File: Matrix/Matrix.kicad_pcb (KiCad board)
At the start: 4 copper layers, 81 x 49.8 mm, 513 parts, among them J1 Conn_02x24_Odd_Even

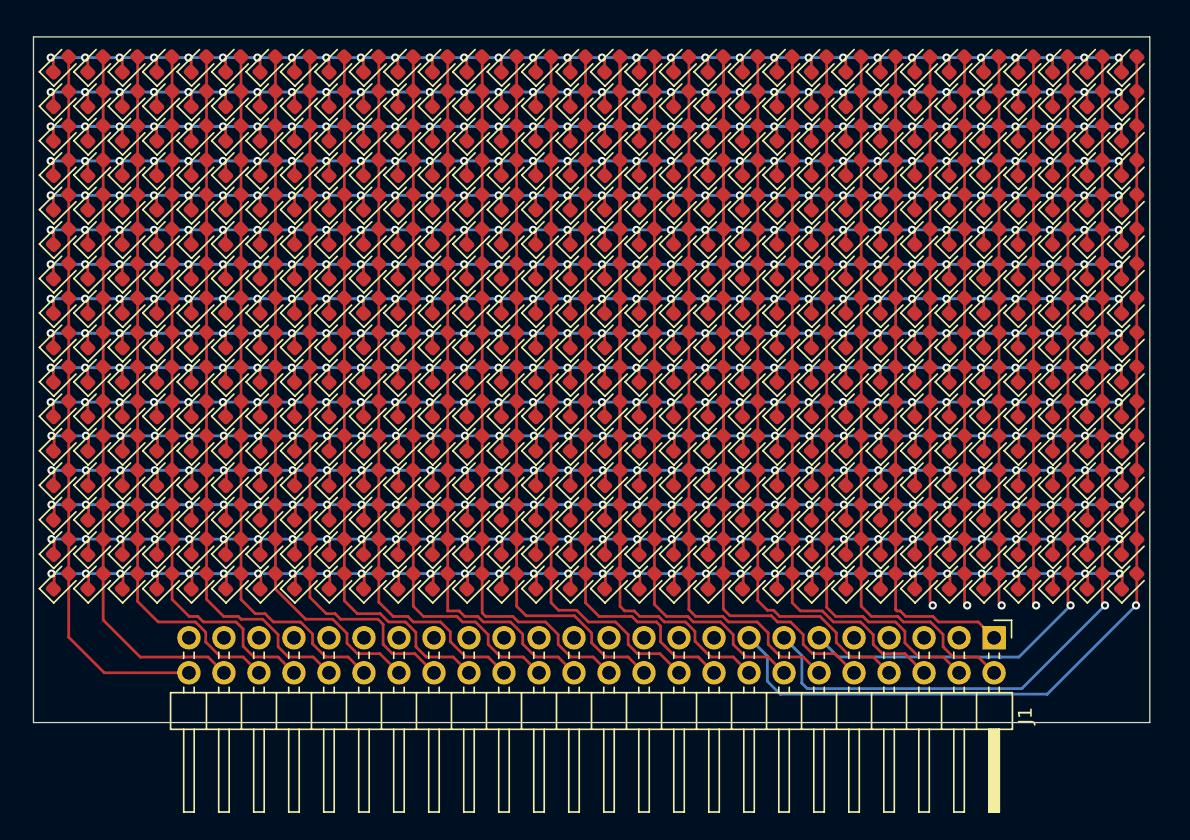
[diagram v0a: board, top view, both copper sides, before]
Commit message: getting ready for another review
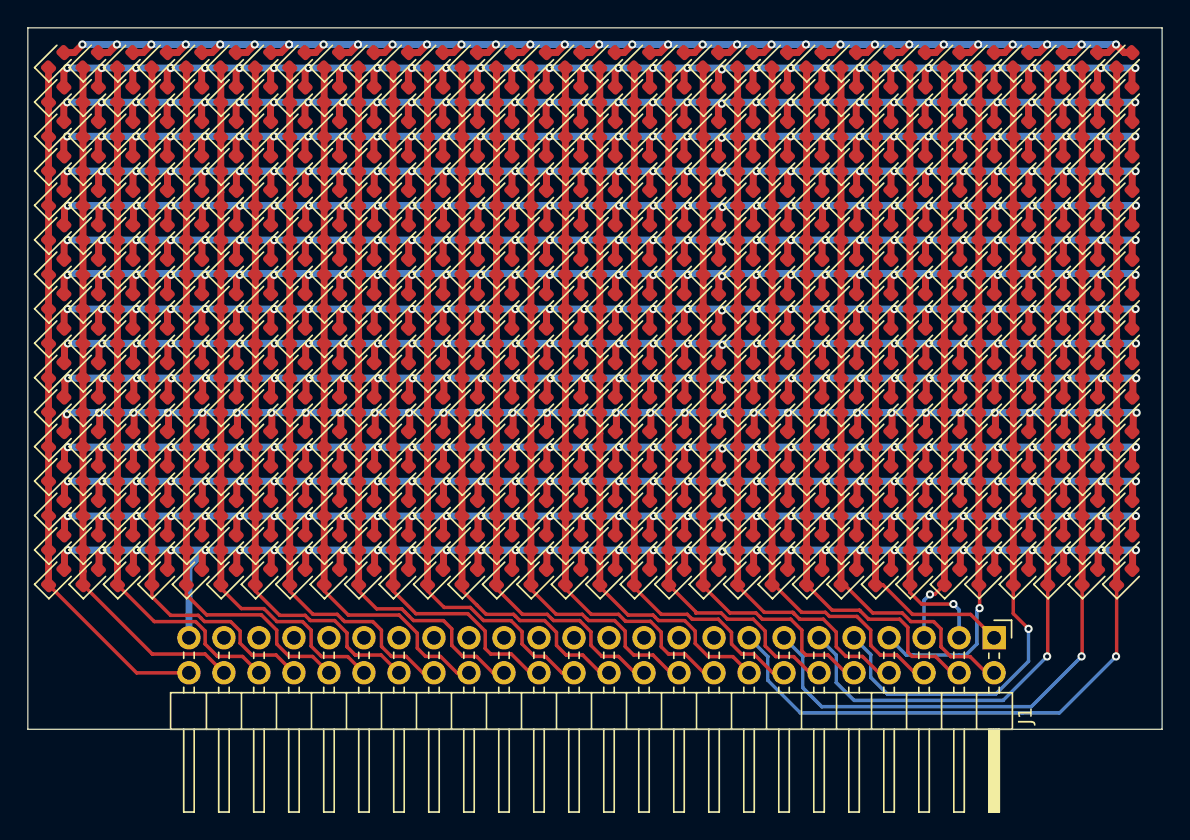
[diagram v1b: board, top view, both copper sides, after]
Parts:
- D1, D10, D100, D101, D102, D103, D104, D105, D106, D107, D108, D109, D11, D110, D111, D112, D113, D114, D115, D116, D117, D118, D119, D12, D120, D121, D122, D123, D124, D125, D126, D127, D128, D129, D13, D130, D131, D132, D133, D134, D135, D136, D137, D138, D139, D14, D140, D141, D142, D143, D144, D145, D146, D147, D148, D149, D15, D150, D151, D152, D153, D154, D155, D156, D157, D158, D159, D16, D160, D161, D162, D163, D164, D165, D166, D167, D168, D169, D17, D170, D171, D172, D173, D174, D175, D176, D177, D178, D179, D18, D180, D181, D182, D183, D184, D185, D186, D187, D188, D189, D19, D190, D191, D192, D193, D194, D195, D196, D197, D198, D199, D2, D20, D200, D201, D202, D203, D204, D205, D206, D207, D208, D209, D21, D210, D211, D212, D213, D214, D215, D216, D217, D218, D219, D22, D220, D221, D222, D223, D224, D225, D226, D227, D228, D229, D23, D230, D231, D232, D233, D234, D235, D236, D237, D238, D239, D24, D240, D241, D242, D243, D244, D245, D246, D247, D248, D249, D25, D250, D251, D252, D253, D254, D255, D256, D257, D258, D259, D26, D260, D261, D262, D263, D264, D265, D266, D267, D268, D269, D27, D270, D271, D272, D273, D274, D275, D276, D277, D278, D279, D28, D280, D281, D282, D283, D284, D285, D286, D287, D288, D289, D29, D290, D291, D292, D293, D294, D295, D296, D297, D298, D299, D3, D30, D300, D301, D302, D303, D304, D305, D306, D307, D308, D309, D31, D310, D311, D312, D313, D314, D315, D316, D317, D318, D319, D32, D320, D321, D322, D323, D324, D325, D326, D327, D328, D329, D33, D330, D331, D332, D333, D334, D335, D336, D337, D338, D339, D34, D340, D341, D342, D343, D344, D345, D346, D347, D348, D349, D35, D350, D351, D352, D353, D354, D355, D356, D357, D358, D359, D36, D360, D361, D362, D363, D364, D365, D366, D367, D368, D369, D37, D370, D371, D372, D373, D374, D375, D376, D377, D378, D379, D38, D380, D381, D382, D383, D384, D385, D386, D387, D388, D389, D39, D390, D391, D392, D393, D394, D395, D396, D397, D398, D399, D4, D40, D400, D401, D402, D403, D404, D405, D406, D407, D408, D409, D41, D410, D411, D412, D413, D414, D415, D416, D417, D418, D419, D42, D420, D421, D422, D423, D424, D425, D426, D427, D428, D429, D43, D430, D431, D432, D433, D434, D435, D436, D437, D438, D439, D44, D440, D441, D442, D443, D444, D445, D446, D447, D448, D449, D45, D450, D451, D452, D453, D454, D455, D456, D457, D458, D459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: value LED -> SML-D12U1WT86
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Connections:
- D10 pad 1: Net-(D10-K) -> Net-(D1-K)
- D10 pad 2: Net-(D1-A) -> Net-(D10-A)
- D101 pad 1: Net-(D101-K) -> Net-(D100-K)
- D101 pad 2: Net-(D100-A) -> Net-(D101-A)
- D102 pad 1: Net-(D102-K) -> Net-(D100-K)
- D102 pad 2: Net-(D100-A) -> Net-(D102-A)
- D103 pad 1: Net-(D103-K) -> Net-(D100-K)
- D103 pad 2: Net-(D100-A) -> Net-(D103-A)
- D104 pad 1: Net-(D104-K) -> Net-(D100-K)
- D104 pad 2: Net-(D100-A) -> Net-(D104-A)
- D105 pad 1: Net-(D105-K) -> Net-(D100-K)
- D105 pad 2: Net-(D100-A) -> Net-(D105-A)
- D106 pad 1: Net-(D10-K) -> Net-(D100-K)
- D106 pad 2: Net-(D100-A) -> Net-(D10-A)
- D107 pad 1: Net-(D107-K) -> Net-(D100-K)
- D107 pad 2: Net-(D100-A) -> Net-(D107-A)
- D108 pad 1: Net-(D108-K) -> Net-(D100-K)
- D108 pad 2: Net-(D100-A) -> Net-(D108-A)
- D109 pad 1: Net-(D109-K) -> Net-(D100-K)
- D109 pad 2: Net-(D100-A) -> Net-(D109-A)
- D11 pad 1: Net-(D107-K) -> Net-(D1-K)
- D11 pad 2: Net-(D1-A) -> Net-(D107-A)
- D110 pad 1: Net-(D110-K) -> Net-(D100-K)
- D110 pad 2: Net-(D100-A) -> Net-(D110-A)
- D111 pad 1: Net-(D111-K) -> Net-(D100-K)
- D111 pad 2: Net-(D100-A) -> Net-(D111-A)
- D112 pad 1: Net-(D112-K) -> Net-(D100-K)
- D112 pad 2: Net-(D100-A) -> Net-(D112-A)
- D113 pad 1: Net-(D1-K) -> Net-(D113-K)
- D113 pad 2: Net-(D113-A) -> Net-(D1-A)
- D114 pad 1: Net-(D114-K) -> Net-(D113-K)
- D114 pad 2: Net-(D113-A) -> Net-(D114-A)
- D115 pad 1: Net-(D115-K) -> Net-(D113-K)
- D115 pad 2: Net-(D113-A) -> Net-(D115-A)
- D116 pad 1: Net-(D100-K) -> Net-(D113-K)
- D116 pad 2: Net-(D113-A) -> Net-(D100-A)
- D117 pad 1: Net-(D101-K) -> Net-(D113-K)
- D117 pad 2: Net-(D113-A) -> Net-(D101-A)
- D118 pad 1: Net-(D102-K) -> Net-(D113-K)
- D118 pad 2: Net-(D113-A) -> Net-(D102-A)
- D119 pad 1: Net-(D103-K) -> Net-(D113-K)
- D119 pad 2: Net-(D113-A) -> Net-(D103-A)
- D12 pad 1: Net-(D108-K) -> Net-(D1-K)
- D12 pad 2: Net-(D1-A) -> Net-(D108-A)
- D120 pad 1: Net-(D104-K) -> Net-(D113-K)
- D120 pad 2: Net-(D113-A) -> Net-(D104-A)
- D121 pad 1: Net-(D105-K) -> Net-(D113-K)
- D121 pad 2: Net-(D113-A) -> Net-(D105-A)
- D122 pad 1: Net-(D10-K) -> Net-(D113-K)
- D122 pad 2: Net-(D113-A) -> Net-(D10-A)
- D123 pad 1: Net-(D107-K) -> Net-(D113-K)
- D123 pad 2: Net-(D113-A) -> Net-(D107-A)
- D124 pad 1: Net-(D108-K) -> Net-(D113-K)
- D124 pad 2: Net-(D113-A) -> Net-(D108-A)
- D125 pad 1: Net-(D109-K) -> Net-(D113-K)
- D125 pad 2: Net-(D113-A) -> Net-(D109-A)
- D126 pad 1: Net-(D110-K) -> Net-(D113-K)
- D126 pad 2: Net-(D113-A) -> Net-(D110-A)
- D127 pad 1: Net-(D111-K) -> Net-(D113-K)
- D127 pad 2: Net-(D113-A) -> Net-(D111-A)
- D128 pad 1: Net-(D112-K) -> Net-(D113-K)
- D128 pad 2: Net-(D113-A) -> Net-(D112-A)
- D129 pad 1: Net-(D1-K) -> Net-(D129-K)
- D129 pad 2: Net-(D129-A) -> Net-(D1-A)
- D13 pad 1: Net-(D109-K) -> Net-(D1-K)
- D13 pad 2: Net-(D1-A) -> Net-(D109-A)
- D130 pad 1: Net-(D114-K) -> Net-(D129-K)
- D130 pad 2: Net-(D129-A) -> Net-(D114-A)
- D131 pad 1: Net-(D115-K) -> Net-(D129-K)
- D131 pad 2: Net-(D129-A) -> Net-(D115-A)
- D132 pad 1: Net-(D100-K) -> Net-(D129-K)
- D132 pad 2: Net-(D129-A) -> Net-(D100-A)
- D133 pad 1: Net-(D101-K) -> Net-(D129-K)
- D133 pad 2: Net-(D129-A) -> Net-(D101-A)
- D134 pad 1: Net-(D102-K) -> Net-(D129-K)
- D134 pad 2: Net-(D129-A) -> Net-(D102-A)
- D135 pad 1: Net-(D103-K) -> Net-(D129-K)
- D135 pad 2: Net-(D129-A) -> Net-(D103-A)
- D136 pad 1: Net-(D104-K) -> Net-(D129-K)
- D136 pad 2: Net-(D129-A) -> Net-(D104-A)
- D137 pad 1: Net-(D105-K) -> Net-(D129-K)
- D137 pad 2: Net-(D129-A) -> Net-(D105-A)
- D138 pad 1: Net-(D10-K) -> Net-(D129-K)
- D138 pad 2: Net-(D129-A) -> Net-(D10-A)
- D139 pad 1: Net-(D107-K) -> Net-(D129-K)
- D139 pad 2: Net-(D129-A) -> Net-(D107-A)
- D14 pad 1: Net-(D110-K) -> Net-(D1-K)
- D14 pad 2: Net-(D1-A) -> Net-(D110-A)
- D140 pad 1: Net-(D108-K) -> Net-(D129-K)
- D140 pad 2: Net-(D129-A) -> Net-(D108-A)
- D141 pad 1: Net-(D109-K) -> Net-(D129-K)
- D141 pad 2: Net-(D129-A) -> Net-(D109-A)
- D142 pad 1: Net-(D110-K) -> Net-(D129-K)
- D142 pad 2: Net-(D129-A) -> Net-(D110-A)
- D143 pad 1: Net-(D111-K) -> Net-(D129-K)
- D143 pad 2: Net-(D129-A) -> Net-(D111-A)
- D144 pad 1: Net-(D112-K) -> Net-(D129-K)
- D144 pad 2: Net-(D129-A) -> Net-(D112-A)
- D145 pad 1: Net-(D1-K) -> Net-(D145-K)
- D145 pad 2: Net-(D145-A) -> Net-(D1-A)
- D146 pad 1: Net-(D114-K) -> Net-(D145-K)
- D146 pad 2: Net-(D145-A) -> Net-(D114-A)
- D147 pad 1: Net-(D115-K) -> Net-(D145-K)
- D147 pad 2: Net-(D145-A) -> Net-(D115-A)
- D148 pad 1: Net-(D100-K) -> Net-(D145-K)
- D148 pad 2: Net-(D145-A) -> Net-(D100-A)
- D149 pad 1: Net-(D101-K) -> Net-(D145-K)
- D149 pad 2: Net-(D145-A) -> Net-(D101-A)
- D15 pad 1: Net-(D111-K) -> Net-(D1-K)
- D15 pad 2: Net-(D1-A) -> Net-(D111-A)
- D150 pad 1: Net-(D102-K) -> Net-(D145-K)
- D150 pad 2: Net-(D145-A) -> Net-(D102-A)
- D151 pad 1: Net-(D103-K) -> Net-(D145-K)
- D151 pad 2: Net-(D145-A) -> Net-(D103-A)
- D152 pad 1: Net-(D104-K) -> Net-(D145-K)
- D152 pad 2: Net-(D145-A) -> Net-(D104-A)
- D153 pad 1: Net-(D105-K) -> Net-(D145-K)
- D153 pad 2: Net-(D145-A) -> Net-(D105-A)
- D154 pad 1: Net-(D10-K) -> Net-(D145-K)
- D154 pad 2: Net-(D145-A) -> Net-(D10-A)
- D155 pad 1: Net-(D107-K) -> Net-(D145-K)
- D155 pad 2: Net-(D145-A) -> Net-(D107-A)
- D156 pad 1: Net-(D108-K) -> Net-(D145-K)
- D156 pad 2: Net-(D145-A) -> Net-(D108-A)
- D157 pad 1: Net-(D109-K) -> Net-(D145-K)
- D157 pad 2: Net-(D145-A) -> Net-(D109-A)
- D158 pad 1: Net-(D110-K) -> Net-(D145-K)
- D158 pad 2: Net-(D145-A) -> Net-(D110-A)
- D159 pad 1: Net-(D111-K) -> Net-(D145-K)
- D159 pad 2: Net-(D145-A) -> Net-(D111-A)
- D16 pad 1: Net-(D112-K) -> Net-(D1-K)
- D16 pad 2: Net-(D1-A) -> Net-(D112-A)
- D160 pad 1: Net-(D112-K) -> Net-(D145-K)
- D160 pad 2: Net-(D145-A) -> Net-(D112-A)
- D161 pad 1: Net-(D1-K) -> Net-(D161-K)
- D161 pad 2: Net-(D161-A) -> Net-(D1-A)
- D162 pad 1: Net-(D114-K) -> Net-(D161-K)
- D162 pad 2: Net-(D161-A) -> Net-(D114-A)
- D163 pad 1: Net-(D115-K) -> Net-(D161-K)
- D163 pad 2: Net-(D161-A) -> Net-(D115-A)
- D164 pad 1: Net-(D100-K) -> Net-(D161-K)
- D164 pad 2: Net-(D161-A) -> Net-(D100-A)
- D165 pad 1: Net-(D101-K) -> Net-(D161-K)
- D165 pad 2: Net-(D161-A) -> Net-(D101-A)
- D166 pad 1: Net-(D102-K) -> Net-(D161-K)
- D166 pad 2: Net-(D161-A) -> Net-(D102-A)
- D167 pad 1: Net-(D103-K) -> Net-(D161-K)
- D167 pad 2: Net-(D161-A) -> Net-(D103-A)
- D168 pad 1: Net-(D104-K) -> Net-(D161-K)
- D168 pad 2: Net-(D161-A) -> Net-(D104-A)
- D169 pad 1: Net-(D105-K) -> Net-(D161-K)
- D169 pad 2: Net-(D161-A) -> Net-(D105-A)
- D17 pad 1: Net-(D1-K) -> Net-(D17-K)
- D17 pad 2: Net-(D17-A) -> Net-(D1-A)
- D170 pad 1: Net-(D10-K) -> Net-(D161-K)
- D170 pad 2: Net-(D161-A) -> Net-(D10-A)
- D171 pad 1: Net-(D107-K) -> Net-(D161-K)
- D171 pad 2: Net-(D161-A) -> Net-(D107-A)
- D172 pad 1: Net-(D108-K) -> Net-(D161-K)
- D172 pad 2: Net-(D161-A) -> Net-(D108-A)
- D173 pad 1: Net-(D109-K) -> Net-(D161-K)
- D173 pad 2: Net-(D161-A) -> Net-(D109-A)
- D174 pad 1: Net-(D110-K) -> Net-(D161-K)
- D174 pad 2: Net-(D161-A) -> Net-(D110-A)
- D175 pad 1: Net-(D111-K) -> Net-(D161-K)
- D175 pad 2: Net-(D161-A) -> Net-(D111-A)
- D176 pad 1: Net-(D112-K) -> Net-(D161-K)
- D176 pad 2: Net-(D161-A) -> Net-(D112-A)
- D177 pad 1: Net-(D1-K) -> Net-(D177-K)
- D177 pad 2: Net-(D177-A) -> Net-(D1-A)
- D178 pad 1: Net-(D114-K) -> Net-(D177-K)
- D178 pad 2: Net-(D177-A) -> Net-(D114-A)
- D179 pad 1: Net-(D115-K) -> Net-(D177-K)
- D179 pad 2: Net-(D177-A) -> Net-(D115-A)
- D18 pad 1: Net-(D114-K) -> Net-(D17-K)
- D18 pad 2: Net-(D17-A) -> Net-(D114-A)
- D180 pad 1: Net-(D100-K) -> Net-(D177-K)
- D180 pad 2: Net-(D177-A) -> Net-(D100-A)
- D181 pad 1: Net-(D101-K) -> Net-(D177-K)
- D181 pad 2: Net-(D177-A) -> Net-(D101-A)
- D182 pad 1: Net-(D102-K) -> Net-(D177-K)
- D182 pad 2: Net-(D177-A) -> Net-(D102-A)
- D183 pad 1: Net-(D103-K) -> Net-(D177-K)
- D183 pad 2: Net-(D177-A) -> Net-(D103-A)
- D184 pad 1: Net-(D104-K) -> Net-(D177-K)
- D184 pad 2: Net-(D177-A) -> Net-(D104-A)
- D185 pad 1: Net-(D105-K) -> Net-(D177-K)
- D185 pad 2: Net-(D177-A) -> Net-(D105-A)
- D186 pad 1: Net-(D10-K) -> Net-(D177-K)
- D186 pad 2: Net-(D177-A) -> Net-(D10-A)
- D187 pad 1: Net-(D107-K) -> Net-(D177-K)
- D187 pad 2: Net-(D177-A) -> Net-(D107-A)
- D188 pad 1: Net-(D108-K) -> Net-(D177-K)
- D188 pad 2: Net-(D177-A) -> Net-(D108-A)
- D189 pad 1: Net-(D109-K) -> Net-(D177-K)
- D189 pad 2: Net-(D177-A) -> Net-(D109-A)
- D19 pad 1: Net-(D115-K) -> Net-(D17-K)
- D19 pad 2: Net-(D17-A) -> Net-(D115-A)
- D190 pad 1: Net-(D110-K) -> Net-(D177-K)
- D190 pad 2: Net-(D177-A) -> Net-(D110-A)
- D191 pad 1: Net-(D111-K) -> Net-(D177-K)
- D191 pad 2: Net-(D177-A) -> Net-(D111-A)
- D192 pad 1: Net-(D112-K) -> Net-(D177-K)
- D192 pad 2: Net-(D177-A) -> Net-(D112-A)
- D193 pad 1: Net-(D1-K) -> Net-(D193-K)
- D193 pad 2: Net-(D193-A) -> Net-(D1-A)
- D194 pad 1: Net-(D114-K) -> Net-(D193-K)
- D194 pad 2: Net-(D193-A) -> Net-(D114-A)
- D195 pad 1: Net-(D115-K) -> Net-(D193-K)
- D195 pad 2: Net-(D193-A) -> Net-(D115-A)
- D196 pad 1: Net-(D100-K) -> Net-(D193-K)
- D196 pad 2: Net-(D193-A) -> Net-(D100-A)
- D197 pad 1: Net-(D101-K) -> Net-(D193-K)
- D197 pad 2: Net-(D193-A) -> Net-(D101-A)
- D198 pad 1: Net-(D102-K) -> Net-(D193-K)
- D198 pad 2: Net-(D193-A) -> Net-(D102-A)
- D199 pad 1: Net-(D103-K) -> Net-(D193-K)
- D199 pad 2: Net-(D193-A) -> Net-(D103-A)
- D2 pad 1: Net-(D114-K) -> Net-(D1-K)
- D2 pad 2: Net-(D1-A) -> Net-(D114-A)
- D20 pad 1: Net-(D100-K) -> Net-(D17-K)
- D20 pad 2: Net-(D17-A) -> Net-(D100-A)
- D200 pad 1: Net-(D104-K) -> Net-(D193-K)
- D200 pad 2: Net-(D193-A) -> Net-(D104-A)
- D201 pad 1: Net-(D105-K) -> Net-(D193-K)
- D201 pad 2: Net-(D193-A) -> Net-(D105-A)
- D202 pad 1: Net-(D10-K) -> Net-(D193-K)
- D202 pad 2: Net-(D193-A) -> Net-(D10-A)
- D203 pad 1: Net-(D107-K) -> Net-(D193-K)
- D203 pad 2: Net-(D193-A) -> Net-(D107-A)
- D204 pad 1: Net-(D108-K) -> Net-(D193-K)
- D204 pad 2: Net-(D193-A) -> Net-(D108-A)
- D205 pad 1: Net-(D109-K) -> Net-(D193-K)
- D205 pad 2: Net-(D193-A) -> Net-(D109-A)
- D206 pad 1: Net-(D110-K) -> Net-(D193-K)
- D206 pad 2: Net-(D193-A) -> Net-(D110-A)
- D207 pad 1: Net-(D111-K) -> Net-(D193-K)
- D207 pad 2: Net-(D193-A) -> Net-(D111-A)
- D208 pad 1: Net-(D112-K) -> Net-(D193-K)
- D208 pad 2: Net-(D193-A) -> Net-(D112-A)
- D209 pad 1: Net-(D1-K) -> Net-(D209-K)
- D209 pad 2: Net-(D209-A) -> Net-(D1-A)
- D21 pad 1: Net-(D101-K) -> Net-(D17-K)
- D21 pad 2: Net-(D17-A) -> Net-(D101-A)
- D210 pad 1: Net-(D114-K) -> Net-(D209-K)
- D210 pad 2: Net-(D209-A) -> Net-(D114-A)
- D211 pad 1: Net-(D115-K) -> Net-(D209-K)
- D211 pad 2: Net-(D209-A) -> Net-(D115-A)
- D212 pad 1: Net-(D100-K) -> Net-(D209-K)
- D212 pad 2: Net-(D209-A) -> Net-(D100-A)
- D213 pad 1: Net-(D101-K) -> Net-(D209-K)
- D213 pad 2: Net-(D209-A) -> Net-(D101-A)
- D214 pad 1: Net-(D102-K) -> Net-(D209-K)
- D214 pad 2: Net-(D209-A) -> Net-(D102-A)
- D215 pad 1: Net-(D103-K) -> Net-(D209-K)
- D215 pad 2: Net-(D209-A) -> Net-(D103-A)
- D216 pad 1: Net-(D104-K) -> Net-(D209-K)
- D216 pad 2: Net-(D209-A) -> Net-(D104-A)
- D217 pad 1: Net-(D105-K) -> Net-(D209-K)
- D217 pad 2: Net-(D209-A) -> Net-(D105-A)
- D218 pad 1: Net-(D10-K) -> Net-(D209-K)
- D218 pad 2: Net-(D209-A) -> Net-(D10-A)
- D219 pad 1: Net-(D107-K) -> Net-(D209-K)
- D219 pad 2: Net-(D209-A) -> Net-(D107-A)
- D22 pad 1: Net-(D102-K) -> Net-(D17-K)
- D22 pad 2: Net-(D17-A) -> Net-(D102-A)
- D220 pad 1: Net-(D108-K) -> Net-(D209-K)
- D220 pad 2: Net-(D209-A) -> Net-(D108-A)
- D221 pad 1: Net-(D109-K) -> Net-(D209-K)
- D221 pad 2: Net-(D209-A) -> Net-(D109-A)
- D222 pad 1: Net-(D110-K) -> Net-(D209-K)
- D222 pad 2: Net-(D209-A) -> Net-(D110-A)
- D223 pad 1: Net-(D111-K) -> Net-(D209-K)
- D223 pad 2: Net-(D209-A) -> Net-(D111-A)
- D224 pad 1: Net-(D112-K) -> Net-(D209-K)
- D224 pad 2: Net-(D209-A) -> Net-(D112-A)
- D225 pad 1: Net-(D1-K) -> Net-(D225-K)
- D225 pad 2: Net-(D225-A) -> Net-(D1-A)
- D226 pad 1: Net-(D114-K) -> Net-(D225-K)
- D226 pad 2: Net-(D225-A) -> Net-(D114-A)
- D227 pad 1: Net-(D115-K) -> Net-(D225-K)
- D227 pad 2: Net-(D225-A) -> Net-(D115-A)
- D228 pad 1: Net-(D100-K) -> Net-(D225-K)
- D228 pad 2: Net-(D225-A) -> Net-(D100-A)
- D229 pad 1: Net-(D101-K) -> Net-(D225-K)
- D229 pad 2: Net-(D225-A) -> Net-(D101-A)
- D23 pad 1: Net-(D103-K) -> Net-(D17-K)
- D23 pad 2: Net-(D17-A) -> Net-(D103-A)
- D230 pad 1: Net-(D102-K) -> Net-(D225-K)
- D230 pad 2: Net-(D225-A) -> Net-(D102-A)
- D231 pad 1: Net-(D103-K) -> Net-(D225-K)
- D231 pad 2: Net-(D225-A) -> Net-(D103-A)
- D232 pad 1: Net-(D104-K) -> Net-(D225-K)
- D232 pad 2: Net-(D225-A) -> Net-(D104-A)
- D233 pad 1: Net-(D105-K) -> Net-(D225-K)
- D233 pad 2: Net-(D225-A) -> Net-(D105-A)
- D234 pad 1: Net-(D10-K) -> Net-(D225-K)
- D234 pad 2: Net-(D225-A) -> Net-(D10-A)
- D235 pad 1: Net-(D107-K) -> Net-(D225-K)
- D235 pad 2: Net-(D225-A) -> Net-(D107-A)
- D236 pad 1: Net-(D108-K) -> Net-(D225-K)
- D236 pad 2: Net-(D225-A) -> Net-(D108-A)
- D237 pad 1: Net-(D109-K) -> Net-(D225-K)
- D237 pad 2: Net-(D225-A) -> Net-(D109-A)
- D238 pad 1: Net-(D110-K) -> Net-(D225-K)
- D238 pad 2: Net-(D225-A) -> Net-(D110-A)
- D239 pad 1: Net-(D111-K) -> Net-(D225-K)
- D239 pad 2: Net-(D225-A) -> Net-(D111-A)
- D24 pad 1: Net-(D104-K) -> Net-(D17-K)
- D24 pad 2: Net-(D17-A) -> Net-(D104-A)
- D240 pad 1: Net-(D112-K) -> Net-(D225-K)
- D240 pad 2: Net-(D225-A) -> Net-(D112-A)
- D241 pad 1: Net-(D1-K) -> Net-(D241-K)
- D241 pad 2: Net-(D241-A) -> Net-(D1-A)
- D242 pad 1: Net-(D114-K) -> Net-(D241-K)
- D242 pad 2: Net-(D241-A) -> Net-(D114-A)
- D243 pad 1: Net-(D115-K) -> Net-(D241-K)
- D243 pad 2: Net-(D241-A) -> Net-(D115-A)
- D244 pad 1: Net-(D100-K) -> Net-(D241-K)
- D244 pad 2: Net-(D241-A) -> Net-(D100-A)
- D245 pad 1: Net-(D101-K) -> Net-(D241-K)
- D245 pad 2: Net-(D241-A) -> Net-(D101-A)
- D246 pad 1: Net-(D102-K) -> Net-(D241-K)
- D246 pad 2: Net-(D241-A) -> Net-(D102-A)
- D247 pad 1: Net-(D103-K) -> Net-(D241-K)
- D247 pad 2: Net-(D241-A) -> Net-(D103-A)
- D248 pad 1: Net-(D104-K) -> Net-(D241-K)
- D248 pad 2: Net-(D241-A) -> Net-(D104-A)
- D249 pad 1: Net-(D105-K) -> Net-(D241-K)
- D249 pad 2: Net-(D241-A) -> Net-(D105-A)
- D25 pad 1: Net-(D105-K) -> Net-(D17-K)
- D25 pad 2: Net-(D17-A) -> Net-(D105-A)
- D250 pad 1: Net-(D10-K) -> Net-(D241-K)
- D250 pad 2: Net-(D241-A) -> Net-(D10-A)
- D251 pad 1: Net-(D107-K) -> Net-(D241-K)
- D251 pad 2: Net-(D241-A) -> Net-(D107-A)
- D252 pad 1: Net-(D108-K) -> Net-(D241-K)
- D252 pad 2: Net-(D241-A) -> Net-(D108-A)
- D253 pad 1: Net-(D109-K) -> Net-(D241-K)
- D253 pad 2: Net-(D241-A) -> Net-(D109-A)
- D254 pad 1: Net-(D110-K) -> Net-(D241-K)
- D254 pad 2: Net-(D241-A) -> Net-(D110-A)
- D255 pad 1: Net-(D111-K) -> Net-(D241-K)
- D255 pad 2: Net-(D241-A) -> Net-(D111-A)
- D256 pad 1: Net-(D112-K) -> Net-(D241-K)
- D256 pad 2: Net-(D241-A) -> Net-(D112-A)
- D257 pad 1: Net-(D1-K) -> Net-(D257-K)
- D257 pad 2: Net-(D257-A) -> Net-(D1-A)
- D258 pad 1: Net-(D114-K) -> Net-(D257-K)
- D258 pad 2: Net-(D257-A) -> Net-(D114-A)
- D259 pad 1: Net-(D115-K) -> Net-(D257-K)
- D259 pad 2: Net-(D257-A) -> Net-(D115-A)
- D26 pad 1: Net-(D10-K) -> Net-(D17-K)
- D26 pad 2: Net-(D17-A) -> Net-(D10-A)
- D260 pad 1: Net-(D100-K) -> Net-(D257-K)
- D260 pad 2: Net-(D257-A) -> Net-(D100-A)
- D261 pad 1: Net-(D101-K) -> Net-(D257-K)
- D261 pad 2: Net-(D257-A) -> Net-(D101-A)
- D262 pad 1: Net-(D102-K) -> Net-(D257-K)
- D262 pad 2: Net-(D257-A) -> Net-(D102-A)
- D263 pad 1: Net-(D103-K) -> Net-(D257-K)
- D263 pad 2: Net-(D257-A) -> Net-(D103-A)
- D264 pad 1: Net-(D104-K) -> Net-(D257-K)
- D264 pad 2: Net-(D257-A) -> Net-(D104-A)
- D265 pad 1: Net-(D105-K) -> Net-(D257-K)
- D265 pad 2: Net-(D257-A) -> Net-(D105-A)
- D266 pad 1: Net-(D10-K) -> Net-(D257-K)
- D266 pad 2: Net-(D257-A) -> Net-(D10-A)
- D267 pad 1: Net-(D107-K) -> Net-(D257-K)
- D267 pad 2: Net-(D257-A) -> Net-(D107-A)
- D268 pad 1: Net-(D108-K) -> Net-(D257-K)
- D268 pad 2: Net-(D257-A) -> Net-(D108-A)
- D269 pad 1: Net-(D109-K) -> Net-(D257-K)
- D269 pad 2: Net-(D257-A) -> Net-(D109-A)
- D27 pad 1: Net-(D107-K) -> Net-(D17-K)
- D27 pad 2: Net-(D17-A) -> Net-(D107-A)
- D270 pad 1: Net-(D110-K) -> Net-(D257-K)
- D270 pad 2: Net-(D257-A) -> Net-(D110-A)
- D271 pad 1: Net-(D111-K) -> Net-(D257-K)
- D271 pad 2: Net-(D257-A) -> Net-(D111-A)
- D272 pad 1: Net-(D112-K) -> Net-(D257-K)
- D272 pad 2: Net-(D257-A) -> Net-(D112-A)
- D273 pad 1: Net-(D1-K) -> Net-(D273-K)
- D273 pad 2: Net-(D273-A) -> Net-(D1-A)
- D274 pad 1: Net-(D114-K) -> Net-(D273-K)
- D274 pad 2: Net-(D273-A) -> Net-(D114-A)
- D275 pad 1: Net-(D115-K) -> Net-(D273-K)
- D275 pad 2: Net-(D273-A) -> Net-(D115-A)
- D276 pad 1: Net-(D100-K) -> Net-(D273-K)
- D276 pad 2: Net-(D273-A) -> Net-(D100-A)
- D277 pad 1: Net-(D101-K) -> Net-(D273-K)
- D277 pad 2: Net-(D273-A) -> Net-(D101-A)
- D278 pad 1: Net-(D102-K) -> Net-(D273-K)
- D278 pad 2: Net-(D273-A) -> Net-(D102-A)
- D279 pad 1: Net-(D103-K) -> Net-(D273-K)
- D279 pad 2: Net-(D273-A) -> Net-(D103-A)
- D28 pad 1: Net-(D108-K) -> Net-(D17-K)
- D28 pad 2: Net-(D17-A) -> Net-(D108-A)
- D280 pad 1: Net-(D104-K) -> Net-(D273-K)
- D280 pad 2: Net-(D273-A) -> Net-(D104-A)
- D281 pad 1: Net-(D105-K) -> Net-(D273-K)
- D281 pad 2: Net-(D273-A) -> Net-(D105-A)
- D282 pad 1: Net-(D10-K) -> Net-(D273-K)
- D282 pad 2: Net-(D273-A) -> Net-(D10-A)
- D283 pad 1: Net-(D107-K) -> Net-(D273-K)
- D283 pad 2: Net-(D273-A) -> Net-(D107-A)
- D284 pad 1: Net-(D108-K) -> Net-(D273-K)
- D284 pad 2: Net-(D273-A) -> Net-(D108-A)
- D285 pad 1: Net-(D109-K) -> Net-(D273-K)
- D285 pad 2: Net-(D273-A) -> Net-(D109-A)
- D286 pad 1: Net-(D110-K) -> Net-(D273-K)
- D286 pad 2: Net-(D273-A) -> Net-(D110-A)
- D287 pad 1: Net-(D111-K) -> Net-(D273-K)
- D287 pad 2: Net-(D273-A) -> Net-(D111-A)
- D288 pad 1: Net-(D112-K) -> Net-(D273-K)
- D288 pad 2: Net-(D273-A) -> Net-(D112-A)
- D289 pad 1: Net-(D1-K) -> Net-(D289-K)
- D289 pad 2: Net-(D289-A) -> Net-(D1-A)
- D29 pad 1: Net-(D109-K) -> Net-(D17-K)
- D29 pad 2: Net-(D17-A) -> Net-(D109-A)
- D290 pad 1: Net-(D114-K) -> Net-(D289-K)
- D290 pad 2: Net-(D289-A) -> Net-(D114-A)
- D291 pad 1: Net-(D115-K) -> Net-(D289-K)
- D291 pad 2: Net-(D289-A) -> Net-(D115-A)
- D292 pad 1: Net-(D100-K) -> Net-(D289-K)
- D292 pad 2: Net-(D289-A) -> Net-(D100-A)
- D293 pad 1: Net-(D101-K) -> Net-(D289-K)
- D293 pad 2: Net-(D289-A) -> Net-(D101-A)
- D294 pad 1: Net-(D102-K) -> Net-(D289-K)
- D294 pad 2: Net-(D289-A) -> Net-(D102-A)
- D295 pad 1: Net-(D103-K) -> Net-(D289-K)
- D295 pad 2: Net-(D289-A) -> Net-(D103-A)
- D296 pad 1: Net-(D104-K) -> Net-(D289-K)
- D296 pad 2: Net-(D289-A) -> Net-(D104-A)
- D297 pad 1: Net-(D105-K) -> Net-(D289-K)
- D297 pad 2: Net-(D289-A) -> Net-(D105-A)
- D298 pad 1: Net-(D10-K) -> Net-(D289-K)
- D298 pad 2: Net-(D289-A) -> Net-(D10-A)
- D299 pad 1: Net-(D107-K) -> Net-(D289-K)
- D299 pad 2: Net-(D289-A) -> Net-(D107-A)
- D3 pad 1: Net-(D115-K) -> Net-(D1-K)
- D3 pad 2: Net-(D1-A) -> Net-(D115-A)
- D30 pad 1: Net-(D110-K) -> Net-(D17-K)
- D30 pad 2: Net-(D17-A) -> Net-(D110-A)
- D300 pad 1: Net-(D108-K) -> Net-(D289-K)
- D300 pad 2: Net-(D289-A) -> Net-(D108-A)
- D301 pad 1: Net-(D109-K) -> Net-(D289-K)
- D301 pad 2: Net-(D289-A) -> Net-(D109-A)
- D302 pad 1: Net-(D110-K) -> Net-(D289-K)
- D302 pad 2: Net-(D289-A) -> Net-(D110-A)
- D303 pad 1: Net-(D111-K) -> Net-(D289-K)
- D303 pad 2: Net-(D289-A) -> Net-(D111-A)
- D304 pad 1: Net-(D112-K) -> Net-(D289-K)
- D304 pad 2: Net-(D289-A) -> Net-(D112-A)
- D305 pad 1: Net-(D1-K) -> Net-(D305-K)
- D305 pad 2: Net-(D305-A) -> Net-(D1-A)
- D306 pad 1: Net-(D114-K) -> Net-(D305-K)
- D306 pad 2: Net-(D305-A) -> Net-(D114-A)
- D307 pad 1: Net-(D115-K) -> Net-(D305-K)
- D307 pad 2: Net-(D305-A) -> Net-(D115-A)
- D308 pad 1: Net-(D100-K) -> Net-(D305-K)
- D308 pad 2: Net-(D305-A) -> Net-(D100-A)
- D309 pad 1: Net-(D101-K) -> Net-(D305-K)
- D309 pad 2: Net-(D305-A) -> Net-(D101-A)
- D31 pad 1: Net-(D111-K) -> Net-(D17-K)
- D31 pad 2: Net-(D17-A) -> Net-(D111-A)
- D310 pad 1: Net-(D102-K) -> Net-(D305-K)
- D310 pad 2: Net-(D305-A) -> Net-(D102-A)
- D311 pad 1: Net-(D103-K) -> Net-(D305-K)
- D311 pad 2: Net-(D305-A) -> Net-(D103-A)
- D312 pad 1: Net-(D104-K) -> Net-(D305-K)
- D312 pad 2: Net-(D305-A) -> Net-(D104-A)
- D313 pad 1: Net-(D105-K) -> Net-(D305-K)
- D313 pad 2: Net-(D305-A) -> Net-(D105-A)
- D314 pad 1: Net-(D10-K) -> Net-(D305-K)
- D314 pad 2: Net-(D305-A) -> Net-(D10-A)
- D315 pad 1: Net-(D107-K) -> Net-(D305-K)
- D315 pad 2: Net-(D305-A) -> Net-(D107-A)
- D316 pad 1: Net-(D108-K) -> Net-(D305-K)
- D316 pad 2: Net-(D305-A) -> Net-(D108-A)
- D317 pad 1: Net-(D109-K) -> Net-(D305-K)
- D317 pad 2: Net-(D305-A) -> Net-(D109-A)
- D318 pad 1: Net-(D110-K) -> Net-(D305-K)
- D318 pad 2: Net-(D305-A) -> Net-(D110-A)
- D319 pad 1: Net-(D111-K) -> Net-(D305-K)
- D319 pad 2: Net-(D305-A) -> Net-(D111-A)
- D32 pad 1: Net-(D112-K) -> Net-(D17-K)
- D32 pad 2: Net-(D17-A) -> Net-(D112-A)
- D320 pad 1: Net-(D112-K) -> Net-(D305-K)
- D320 pad 2: Net-(D305-A) -> Net-(D112-A)
- D321 pad 1: Net-(D1-K) -> Net-(D321-K)
- D321 pad 2: Net-(D321-A) -> Net-(D1-A)
- D322 pad 1: Net-(D114-K) -> Net-(D321-K)
- D322 pad 2: Net-(D321-A) -> Net-(D114-A)
- D323 pad 1: Net-(D115-K) -> Net-(D321-K)
- D323 pad 2: Net-(D321-A) -> Net-(D115-A)
- D324 pad 1: Net-(D100-K) -> Net-(D321-K)
- D324 pad 2: Net-(D321-A) -> Net-(D100-A)
- D325 pad 1: Net-(D101-K) -> Net-(D321-K)
- D325 pad 2: Net-(D321-A) -> Net-(D101-A)
- D326 pad 1: Net-(D102-K) -> Net-(D321-K)
- D326 pad 2: Net-(D321-A) -> Net-(D102-A)
- D327 pad 1: Net-(D103-K) -> Net-(D321-K)
- D327 pad 2: Net-(D321-A) -> Net-(D103-A)
- D328 pad 1: Net-(D104-K) -> Net-(D321-K)
- D328 pad 2: Net-(D321-A) -> Net-(D104-A)
- D329 pad 1: Net-(D105-K) -> Net-(D321-K)
- D329 pad 2: Net-(D321-A) -> Net-(D105-A)
- D33 pad 1: Net-(D1-K) -> Net-(D33-K)
- D33 pad 2: Net-(D33-A) -> Net-(D1-A)
- D330 pad 1: Net-(D10-K) -> Net-(D321-K)
- D330 pad 2: Net-(D321-A) -> Net-(D10-A)
- D331 pad 1: Net-(D107-K) -> Net-(D321-K)
- D331 pad 2: Net-(D321-A) -> Net-(D107-A)
- D332 pad 1: Net-(D108-K) -> Net-(D321-K)
- D332 pad 2: Net-(D321-A) -> Net-(D108-A)
- D333 pad 1: Net-(D109-K) -> Net-(D321-K)
- D333 pad 2: Net-(D321-A) -> Net-(D109-A)
- D334 pad 1: Net-(D110-K) -> Net-(D321-K)
- D334 pad 2: Net-(D321-A) -> Net-(D110-A)
- D335 pad 1: Net-(D111-K) -> Net-(D321-K)
- D335 pad 2: Net-(D321-A) -> Net-(D111-A)
- D336 pad 1: Net-(D112-K) -> Net-(D321-K)
- D336 pad 2: Net-(D321-A) -> Net-(D112-A)
- D337 pad 1: Net-(D1-K) -> Net-(D337-K)
- D337 pad 2: Net-(D337-A) -> Net-(D1-A)
- D338 pad 1: Net-(D114-K) -> Net-(D337-K)
- D338 pad 2: Net-(D337-A) -> Net-(D114-A)
- D339 pad 1: Net-(D115-K) -> Net-(D337-K)
- D339 pad 2: Net-(D337-A) -> Net-(D115-A)
- D34 pad 1: Net-(D114-K) -> Net-(D33-K)
- D34 pad 2: Net-(D33-A) -> Net-(D114-A)
- D340 pad 1: Net-(D100-K) -> Net-(D337-K)
- D340 pad 2: Net-(D337-A) -> Net-(D100-A)
- D341 pad 1: Net-(D101-K) -> Net-(D337-K)
- D341 pad 2: Net-(D337-A) -> Net-(D101-A)
- D342 pad 1: Net-(D102-K) -> Net-(D337-K)
- D342 pad 2: Net-(D337-A) -> Net-(D102-A)
- D343 pad 1: Net-(D103-K) -> Net-(D337-K)
- D343 pad 2: Net-(D337-A) -> Net-(D103-A)
- D344 pad 1: Net-(D104-K) -> Net-(D337-K)
- D344 pad 2: Net-(D337-A) -> Net-(D104-A)
- D345 pad 1: Net-(D105-K) -> Net-(D337-K)
- D345 pad 2: Net-(D337-A) -> Net-(D105-A)
- D346 pad 1: Net-(D10-K) -> Net-(D337-K)
- D346 pad 2: Net-(D337-A) -> Net-(D10-A)
- D347 pad 1: Net-(D107-K) -> Net-(D337-K)
- D347 pad 2: Net-(D337-A) -> Net-(D107-A)
- D348 pad 1: Net-(D108-K) -> Net-(D337-K)
- D348 pad 2: Net-(D337-A) -> Net-(D108-A)
- D349 pad 1: Net-(D109-K) -> Net-(D337-K)
- D349 pad 2: Net-(D337-A) -> Net-(D109-A)
- D35 pad 1: Net-(D115-K) -> Net-(D33-K)
- D35 pad 2: Net-(D33-A) -> Net-(D115-A)
- D350 pad 1: Net-(D110-K) -> Net-(D337-K)
- D350 pad 2: Net-(D337-A) -> Net-(D110-A)
- D351 pad 1: Net-(D111-K) -> Net-(D337-K)
- D351 pad 2: Net-(D337-A) -> Net-(D111-A)
- D352 pad 1: Net-(D112-K) -> Net-(D337-K)
- D352 pad 2: Net-(D337-A) -> Net-(D112-A)
- D353 pad 1: Net-(D1-K) -> Net-(D353-K)
- D353 pad 2: Net-(D353-A) -> Net-(D1-A)
- D354 pad 1: Net-(D114-K) -> Net-(D353-K)
- D354 pad 2: Net-(D353-A) -> Net-(D114-A)
- D355 pad 1: Net-(D115-K) -> Net-(D353-K)
- D355 pad 2: Net-(D353-A) -> Net-(D115-A)
- D356 pad 1: Net-(D100-K) -> Net-(D353-K)
- D356 pad 2: Net-(D353-A) -> Net-(D100-A)
- D357 pad 1: Net-(D101-K) -> Net-(D353-K)
- D357 pad 2: Net-(D353-A) -> Net-(D101-A)
- D358 pad 1: Net-(D102-K) -> Net-(D353-K)
- D358 pad 2: Net-(D353-A) -> Net-(D102-A)
- D359 pad 1: Net-(D103-K) -> Net-(D353-K)
- D359 pad 2: Net-(D353-A) -> Net-(D103-A)
- D36 pad 1: Net-(D100-K) -> Net-(D33-K)
- D36 pad 2: Net-(D33-A) -> Net-(D100-A)
- D360 pad 1: Net-(D104-K) -> Net-(D353-K)
- D360 pad 2: Net-(D353-A) -> Net-(D104-A)
- D361 pad 1: Net-(D105-K) -> Net-(D353-K)
- D361 pad 2: Net-(D353-A) -> Net-(D105-A)
- D362 pad 1: Net-(D10-K) -> Net-(D353-K)
- D362 pad 2: Net-(D353-A) -> Net-(D10-A)
- D363 pad 1: Net-(D107-K) -> Net-(D353-K)
- D363 pad 2: Net-(D353-A) -> Net-(D107-A)
- D364 pad 1: Net-(D108-K) -> Net-(D353-K)
- D364 pad 2: Net-(D353-A) -> Net-(D108-A)
- D365 pad 1: Net-(D109-K) -> Net-(D353-K)
- D365 pad 2: Net-(D353-A) -> Net-(D109-A)
- D366 pad 1: Net-(D110-K) -> Net-(D353-K)
- D366 pad 2: Net-(D353-A) -> Net-(D110-A)
- D367 pad 1: Net-(D111-K) -> Net-(D353-K)
- D367 pad 2: Net-(D353-A) -> Net-(D111-A)
- D368 pad 1: Net-(D112-K) -> Net-(D353-K)
- D368 pad 2: Net-(D353-A) -> Net-(D112-A)
- D369 pad 1: Net-(D1-K) -> Net-(D369-K)
- D369 pad 2: Net-(D369-A) -> Net-(D1-A)
- D37 pad 1: Net-(D101-K) -> Net-(D33-K)
- D37 pad 2: Net-(D33-A) -> Net-(D101-A)
- D370 pad 1: Net-(D114-K) -> Net-(D369-K)
- D370 pad 2: Net-(D369-A) -> Net-(D114-A)
- D371 pad 1: Net-(D115-K) -> Net-(D369-K)
- D371 pad 2: Net-(D369-A) -> Net-(D115-A)
- D372 pad 1: Net-(D100-K) -> Net-(D369-K)
- D372 pad 2: Net-(D369-A) -> Net-(D100-A)
- D373 pad 1: Net-(D101-K) -> Net-(D369-K)
- D373 pad 2: Net-(D369-A) -> Net-(D101-A)
- D374 pad 1: Net-(D102-K) -> Net-(D369-K)
- D374 pad 2: Net-(D369-A) -> Net-(D102-A)
- D375 pad 1: Net-(D103-K) -> Net-(D369-K)
- D375 pad 2: Net-(D369-A) -> Net-(D103-A)
- D376 pad 1: Net-(D104-K) -> Net-(D369-K)
- D376 pad 2: Net-(D369-A) -> Net-(D104-A)
- D377 pad 1: Net-(D105-K) -> Net-(D369-K)
- D377 pad 2: Net-(D369-A) -> Net-(D105-A)
- D378 pad 1: Net-(D10-K) -> Net-(D369-K)
- D378 pad 2: Net-(D369-A) -> Net-(D10-A)
- D379 pad 1: Net-(D107-K) -> Net-(D369-K)
- D379 pad 2: Net-(D369-A) -> Net-(D107-A)
- D38 pad 1: Net-(D102-K) -> Net-(D33-K)
- D38 pad 2: Net-(D33-A) -> Net-(D102-A)
- D380 pad 1: Net-(D108-K) -> Net-(D369-K)
- D380 pad 2: Net-(D369-A) -> Net-(D108-A)
- D381 pad 1: Net-(D109-K) -> Net-(D369-K)
- D381 pad 2: Net-(D369-A) -> Net-(D109-A)
- D382 pad 1: Net-(D110-K) -> Net-(D369-K)
- D382 pad 2: Net-(D369-A) -> Net-(D110-A)
- D383 pad 1: Net-(D111-K) -> Net-(D369-K)
- D383 pad 2: Net-(D369-A) -> Net-(D111-A)
- D384 pad 1: Net-(D112-K) -> Net-(D369-K)
- D384 pad 2: Net-(D369-A) -> Net-(D112-A)
- D385 pad 1: Net-(D1-K) -> Net-(D385-K)
- D385 pad 2: Net-(D385-A) -> Net-(D1-A)
- D386 pad 1: Net-(D114-K) -> Net-(D385-K)
- D386 pad 2: Net-(D385-A) -> Net-(D114-A)
- D387 pad 1: Net-(D115-K) -> Net-(D385-K)
- D387 pad 2: Net-(D385-A) -> Net-(D115-A)
- D388 pad 1: Net-(D100-K) -> Net-(D385-K)
- D388 pad 2: Net-(D385-A) -> Net-(D100-A)
- D389 pad 1: Net-(D101-K) -> Net-(D385-K)
- D389 pad 2: Net-(D385-A) -> Net-(D101-A)
- D39 pad 1: Net-(D103-K) -> Net-(D33-K)
- D39 pad 2: Net-(D33-A) -> Net-(D103-A)
- D390 pad 1: Net-(D102-K) -> Net-(D385-K)
- D390 pad 2: Net-(D385-A) -> Net-(D102-A)
- D391 pad 1: Net-(D103-K) -> Net-(D385-K)
- D391 pad 2: Net-(D385-A) -> Net-(D103-A)
- D392 pad 1: Net-(D104-K) -> Net-(D385-K)
- D392 pad 2: Net-(D385-A) -> Net-(D104-A)
- D393 pad 1: Net-(D105-K) -> Net-(D385-K)
- D393 pad 2: Net-(D385-A) -> Net-(D105-A)
- D394 pad 1: Net-(D10-K) -> Net-(D385-K)
- D394 pad 2: Net-(D385-A) -> Net-(D10-A)
- D395 pad 1: Net-(D107-K) -> Net-(D385-K)
- D395 pad 2: Net-(D385-A) -> Net-(D107-A)
- D396 pad 1: Net-(D108-K) -> Net-(D385-K)
- D396 pad 2: Net-(D385-A) -> Net-(D108-A)
- D397 pad 1: Net-(D109-K) -> Net-(D385-K)
- D397 pad 2: Net-(D385-A) -> Net-(D109-A)
- D398 pad 1: Net-(D110-K) -> Net-(D385-K)
- D398 pad 2: Net-(D385-A) -> Net-(D110-A)
- D399 pad 1: Net-(D111-K) -> Net-(D385-K)
- D399 pad 2: Net-(D385-A) -> Net-(D111-A)
- D4 pad 1: Net-(D100-K) -> Net-(D1-K)
- D4 pad 2: Net-(D1-A) -> Net-(D100-A)
- D40 pad 1: Net-(D104-K) -> Net-(D33-K)
- D40 pad 2: Net-(D33-A) -> Net-(D104-A)
- D400 pad 1: Net-(D112-K) -> Net-(D385-K)
- D400 pad 2: Net-(D385-A) -> Net-(D112-A)
- D401 pad 1: Net-(D1-K) -> Net-(D401-K)
- D401 pad 2: Net-(D401-A) -> Net-(D1-A)
- D402 pad 1: Net-(D114-K) -> Net-(D401-K)
- D402 pad 2: Net-(D401-A) -> Net-(D114-A)
- D403 pad 1: Net-(D115-K) -> Net-(D401-K)
- D403 pad 2: Net-(D401-A) -> Net-(D115-A)
- D404 pad 1: Net-(D100-K) -> Net-(D401-K)
- D404 pad 2: Net-(D401-A) -> Net-(D100-A)
- D405 pad 1: Net-(D101-K) -> Net-(D401-K)
- D405 pad 2: Net-(D401-A) -> Net-(D101-A)
- D406 pad 1: Net-(D102-K) -> Net-(D401-K)
- D406 pad 2: Net-(D401-A) -> Net-(D102-A)
- D407 pad 1: Net-(D103-K) -> Net-(D401-K)
- D407 pad 2: Net-(D401-A) -> Net-(D103-A)
- D408 pad 1: Net-(D104-K) -> Net-(D401-K)
- D408 pad 2: Net-(D401-A) -> Net-(D104-A)
- D409 pad 1: Net-(D105-K) -> Net-(D401-K)
- D409 pad 2: Net-(D401-A) -> Net-(D105-A)
- D41 pad 1: Net-(D105-K) -> Net-(D33-K)
- D41 pad 2: Net-(D33-A) -> Net-(D105-A)
- D410 pad 1: Net-(D10-K) -> Net-(D401-K)
- D410 pad 2: Net-(D401-A) -> Net-(D10-A)
- D411 pad 1: Net-(D107-K) -> Net-(D401-K)
- D411 pad 2: Net-(D401-A) -> Net-(D107-A)
- D412 pad 1: Net-(D108-K) -> Net-(D401-K)
- D412 pad 2: Net-(D401-A) -> Net-(D108-A)
- D413 pad 1: Net-(D109-K) -> Net-(D401-K)
- D413 pad 2: Net-(D401-A) -> Net-(D109-A)
- D414 pad 1: Net-(D110-K) -> Net-(D401-K)
- D414 pad 2: Net-(D401-A) -> Net-(D110-A)
- D415 pad 1: Net-(D111-K) -> Net-(D401-K)
- D415 pad 2: Net-(D401-A) -> Net-(D111-A)
- D416 pad 1: Net-(D112-K) -> Net-(D401-K)
- D416 pad 2: Net-(D401-A) -> Net-(D112-A)
- D417 pad 1: Net-(D1-K) -> Net-(D417-K)
- D417 pad 2: Net-(D417-A) -> Net-(D1-A)
- D418 pad 1: Net-(D114-K) -> Net-(D417-K)
- D418 pad 2: Net-(D417-A) -> Net-(D114-A)
- D419 pad 1: Net-(D115-K) -> Net-(D417-K)
- D419 pad 2: Net-(D417-A) -> Net-(D115-A)
- D42 pad 1: Net-(D10-K) -> Net-(D33-K)
- D42 pad 2: Net-(D33-A) -> Net-(D10-A)
- D420 pad 1: Net-(D100-K) -> Net-(D417-K)
- D420 pad 2: Net-(D417-A) -> Net-(D100-A)
- D421 pad 1: Net-(D101-K) -> Net-(D417-K)
- D421 pad 2: Net-(D417-A) -> Net-(D101-A)
- D422 pad 1: Net-(D102-K) -> Net-(D417-K)
- D422 pad 2: Net-(D417-A) -> Net-(D102-A)
- D423 pad 1: Net-(D103-K) -> Net-(D417-K)
- D423 pad 2: Net-(D417-A) -> Net-(D103-A)
- D424 pad 1: Net-(D104-K) -> Net-(D417-K)
- D424 pad 2: Net-(D417-A) -> Net-(D104-A)
- D425 pad 1: Net-(D105-K) -> Net-(D417-K)
- D425 pad 2: Net-(D417-A) -> Net-(D105-A)
- D426 pad 1: Net-(D10-K) -> Net-(D417-K)
- D426 pad 2: Net-(D417-A) -> Net-(D10-A)
- D427 pad 1: Net-(D107-K) -> Net-(D417-K)
- D427 pad 2: Net-(D417-A) -> Net-(D107-A)
- D428 pad 1: Net-(D108-K) -> Net-(D417-K)
- D428 pad 2: Net-(D417-A) -> Net-(D108-A)
- D429 pad 1: Net-(D109-K) -> Net-(D417-K)
- D429 pad 2: Net-(D417-A) -> Net-(D109-A)
- D43 pad 1: Net-(D107-K) -> Net-(D33-K)
- D43 pad 2: Net-(D33-A) -> Net-(D107-A)
- D430 pad 1: Net-(D110-K) -> Net-(D417-K)
- D430 pad 2: Net-(D417-A) -> Net-(D110-A)
- D431 pad 1: Net-(D111-K) -> Net-(D417-K)
- D431 pad 2: Net-(D417-A) -> Net-(D111-A)
- D432 pad 1: Net-(D112-K) -> Net-(D417-K)
- D432 pad 2: Net-(D417-A) -> Net-(D112-A)
- D433 pad 1: Net-(D1-K) -> Net-(D433-K)
- D433 pad 2: Net-(D433-A) -> Net-(D1-A)
- D434 pad 1: Net-(D114-K) -> Net-(D433-K)
- D434 pad 2: Net-(D433-A) -> Net-(D114-A)
- D435 pad 1: Net-(D115-K) -> Net-(D433-K)
- D435 pad 2: Net-(D433-A) -> Net-(D115-A)
- D436 pad 1: Net-(D100-K) -> Net-(D433-K)
- D436 pad 2: Net-(D433-A) -> Net-(D100-A)
- D437 pad 1: Net-(D101-K) -> Net-(D433-K)
- D437 pad 2: Net-(D433-A) -> Net-(D101-A)
- D438 pad 1: Net-(D102-K) -> Net-(D433-K)
- D438 pad 2: Net-(D433-A) -> Net-(D102-A)
- D439 pad 1: Net-(D103-K) -> Net-(D433-K)
- D439 pad 2: Net-(D433-A) -> Net-(D103-A)
- D44 pad 1: Net-(D108-K) -> Net-(D33-K)
- D44 pad 2: Net-(D33-A) -> Net-(D108-A)
- D440 pad 1: Net-(D104-K) -> Net-(D433-K)
- D440 pad 2: Net-(D433-A) -> Net-(D104-A)
- D441 pad 1: Net-(D105-K) -> Net-(D433-K)
- D441 pad 2: Net-(D433-A) -> Net-(D105-A)
- D442 pad 1: Net-(D10-K) -> Net-(D433-K)
- D442 pad 2: Net-(D433-A) -> Net-(D10-A)
- D443 pad 1: Net-(D107-K) -> Net-(D433-K)
- D443 pad 2: Net-(D433-A) -> Net-(D107-A)
- D444 pad 1: Net-(D108-K) -> Net-(D433-K)
- D444 pad 2: Net-(D433-A) -> Net-(D108-A)
- D445 pad 1: Net-(D109-K) -> Net-(D433-K)
- D445 pad 2: Net-(D433-A) -> Net-(D109-A)
- D446 pad 1: Net-(D110-K) -> Net-(D433-K)
- D446 pad 2: Net-(D433-A) -> Net-(D110-A)
- D447 pad 1: Net-(D111-K) -> Net-(D433-K)
- D447 pad 2: Net-(D433-A) -> Net-(D111-A)
- D448 pad 1: Net-(D112-K) -> Net-(D433-K)
- D448 pad 2: Net-(D433-A) -> Net-(D112-A)
- D449 pad 1: Net-(D1-K) -> Net-(D449-K)
- D449 pad 2: Net-(D449-A) -> Net-(D1-A)
- D45 pad 1: Net-(D109-K) -> Net-(D33-K)
- D45 pad 2: Net-(D33-A) -> Net-(D109-A)
- D450 pad 1: Net-(D114-K) -> Net-(D449-K)
- D450 pad 2: Net-(D449-A) -> Net-(D114-A)
- D451 pad 1: Net-(D115-K) -> Net-(D449-K)
- D451 pad 2: Net-(D449-A) -> Net-(D115-A)
- D452 pad 1: Net-(D100-K) -> Net-(D449-K)
- D452 pad 2: Net-(D449-A) -> Net-(D100-A)
- D453 pad 1: Net-(D101-K) -> Net-(D449-K)
- D453 pad 2: Net-(D449-A) -> Net-(D101-A)
- D454 pad 1: Net-(D102-K) -> Net-(D449-K)
- D454 pad 2: Net-(D449-A) -> Net-(D102-A)
- D455 pad 1: Net-(D103-K) -> Net-(D449-K)
- D455 pad 2: Net-(D449-A) -> Net-(D103-A)
- D456 pad 1: Net-(D104-K) -> Net-(D449-K)
- D456 pad 2: Net-(D449-A) -> Net-(D104-A)
- D457 pad 1: Net-(D105-K) -> Net-(D449-K)
- D457 pad 2: Net-(D449-A) -> Net-(D105-A)
- D458 pad 1: Net-(D10-K) -> Net-(D449-K)
- D458 pad 2: Net-(D449-A) -> Net-(D10-A)
- D459 pad 1: Net-(D107-K) -> Net-(D449-K)
- D459 pad 2: Net-(D449-A) -> Net-(D107-A)
- D46 pad 1: Net-(D110-K) -> Net-(D33-K)
- D46 pad 2: Net-(D33-A) -> Net-(D110-A)
- D460 pad 1: Net-(D108-K) -> Net-(D449-K)
- D460 pad 2: Net-(D449-A) -> Net-(D108-A)
- D461 pad 1: Net-(D109-K) -> Net-(D449-K)
- D461 pad 2: Net-(D449-A) -> Net-(D109-A)
- D462 pad 1: Net-(D110-K) -> Net-(D449-K)
- D462 pad 2: Net-(D449-A) -> Net-(D110-A)
- D463 pad 1: Net-(D111-K) -> Net-(D449-K)
- D463 pad 2: Net-(D449-A) -> Net-(D111-A)
- D464 pad 1: Net-(D112-K) -> Net-(D449-K)
- D464 pad 2: Net-(D449-A) -> Net-(D112-A)
- D465 pad 1: Net-(D1-K) -> Net-(D465-K)
- D465 pad 2: Net-(D465-A) -> Net-(D1-A)
- D466 pad 1: Net-(D114-K) -> Net-(D465-K)
- D466 pad 2: Net-(D465-A) -> Net-(D114-A)
- D467 pad 1: Net-(D115-K) -> Net-(D465-K)
- D467 pad 2: Net-(D465-A) -> Net-(D115-A)
- D468 pad 1: Net-(D100-K) -> Net-(D465-K)
- D468 pad 2: Net-(D465-A) -> Net-(D100-A)
- D469 pad 1: Net-(D101-K) -> Net-(D465-K)
- D469 pad 2: Net-(D465-A) -> Net-(D101-A)
- D47 pad 1: Net-(D111-K) -> Net-(D33-K)
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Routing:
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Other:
- board size 81 x 49.8 mm -> 82.3 x 50.9 mm
